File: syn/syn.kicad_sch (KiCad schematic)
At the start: 47 parts, among them J1 AudioJack2, Q1 BC546, SW1 Range, SW3 Wave, SW4 Wave, SW5 Mod, SW6 SW_Push_SPDT, U1 TL074, U2 LM741

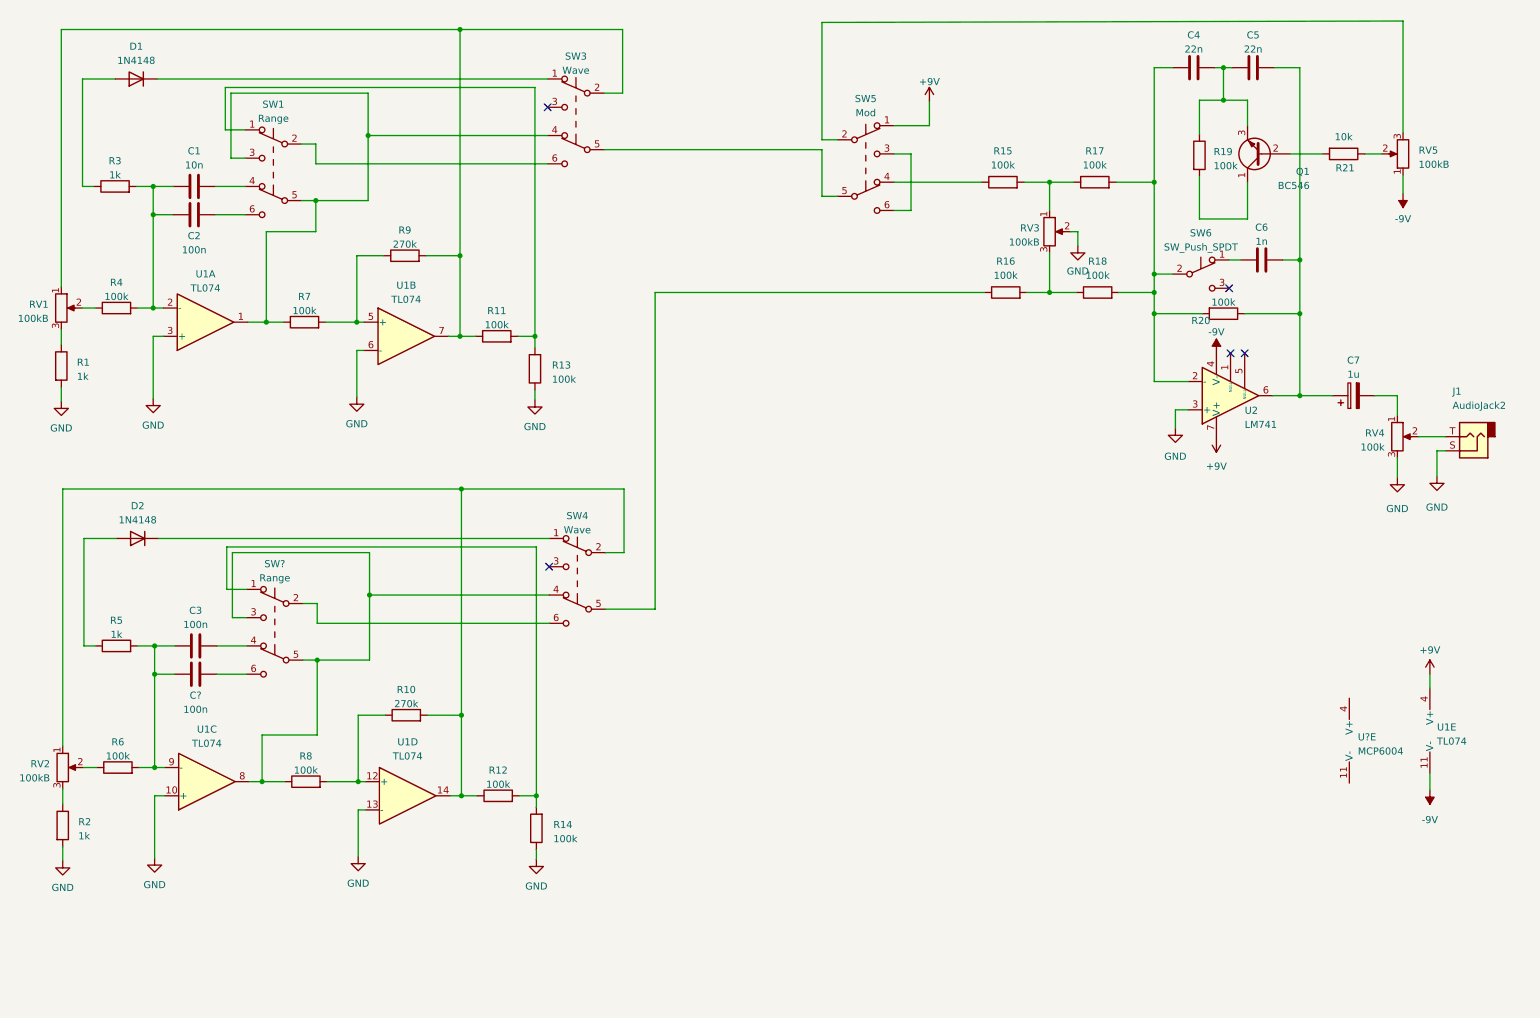
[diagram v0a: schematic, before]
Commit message: structure
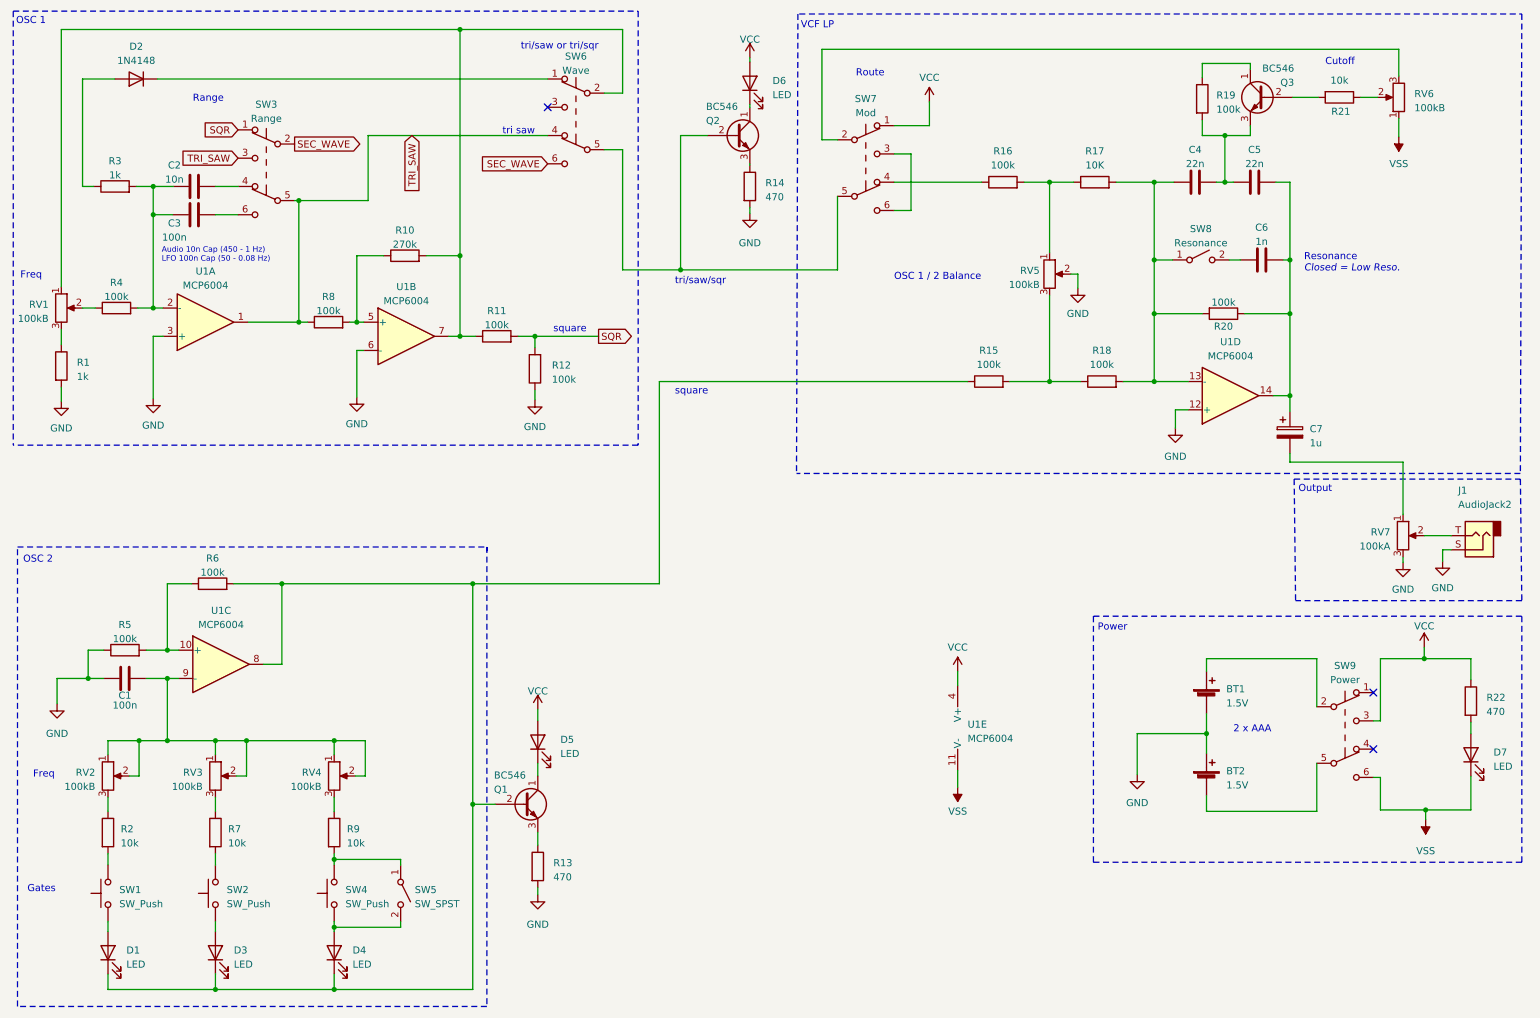
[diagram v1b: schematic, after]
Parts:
- removed C3, C?: 100n, symbol Device:C
- removed D2: 1N4148, Diode_THT:D_DO-35_SOD27_P7.62mm_Horizontal, symbol Diode:1N4148
- removed R10: 270k, symbol Device:R
- removed R12, R8: 100k, symbol Device:R
- removed SW4: Wave, symbol Switch:SW_Push_DPDT
- removed SW6: SW_Push_SPDT, symbol Switch:SW_Push_SPDT
- removed SW?: Range, symbol Switch:SW_Push_DPDT
- removed U1: TL074, symbol Amplifier_Operational:TL074
- removed U2: LM741, symbol Amplifier_Operational:LM741
- removed U?: MCP6004, symbol Amplifier_Operational:MCP6004
- added BT1, BT2: 1.5V, Battery:BatteryHolder_Keystone_2466_1xAAA, symbol Device:Battery_Cell
- added C1: 100n, symbol Device:C
- added D1, D3, D4, D5, D6, D7: LED, symbol Device:LED
- added Q1, Q2: BC546, Package_TO_SOT_THT:TO-92_Inline, symbol Transistor_BJT:BC546
- added R13, R22: 470, symbol Device:R
- added R7, R9: 10k, symbol Device:R
- added RV3, RV4: 100kB, symbol Device:R_Potentiometer
- added SW1, SW2, SW4: SW_Push, symbol Switch:SW_Push
- added SW5: SW_SPST, symbol Switch:SW_SPST
- added SW8: Resonance, symbol Switch:SW_SPST
- added SW9: Power, symbol Switch:SW_Push_DPDT
- added U1: MCP6004, symbol Amplifier_Operational:MCP6004
- R14: value 100k -> 470
- R17: value 100k -> 10K
- R2: value 1k -> 10k
- R5: value 1k -> 100k
- RV7: renamed from RV4; value 100k -> 100kA
- renumbered C1 to C2, C2 to C3, D1 to D2, Q1 to Q3, R9 to R10, R13 to R12, R16 to R15, R15 to R16, R7 to R8, RV3 to RV5, RV5 to RV6, SW1 to SW3, SW3 to SW6, SW5 to SW7
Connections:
- net GND: now also R14.2, R5.1, BT1.2 (-), BT2.1 (+), C1.1, R13.2, U1.12 (+), U1.3 (+), U1.6 (-); no longer R14.1, R2.2
- net at C2.1, C3.1, R3.2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: now also U1.2 (-)
- net TRI_SAW: now reaches R8.1, SW3.3 (C), SW3.5 (B), SW6.4 (A)
- net TRI_SAW: now also U1.1
- net at R5.2: now also R6.1, U1.10 (+); no longer R6.2
- net at C6.1: now also SW8.2 (B)
- net at C5.2, C6.2, C7.1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: now also U1.14
- net at RV2.1: now also RV2.2, C1.2, RV3.1, RV3.2, RV4.1, RV4.2, U1.9 (-)
- net at C4.1, R17.2, R18.2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: now also SW8.1 (A), U1.13 (-)
- net at R10.1, R8.2: now also U1.5 (+)
- net at R10.2, R11.1, RV1.1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: now also U1.7
- net at R15.1: now also R6.2, D1.1 (K), D3.1 (K), D4.1 (K), Q1.2 (B), U1.8
- net at SW6.5 (B), SW7.5 (B): now also Q2.2 (B)
- net SEC_WAVE: now reaches SW3.2 (B), SW6.6 (C)
- net SQR: now reaches R11.2, R12.2, SW3.1 (A)
- net at C4.2, C5.1, Q3.3 (E): now also R19.2; no longer R19.1
- net at Q3.1 (C): now also R19.1; no longer R19.2
- net +9V renamed VCC
- net VCC: now also D5.2 (A), D6.2 (A), R22.1, SW9.3 (C), U1.4 (V+)
- net -9V renamed VSS
- net VSS: now also D7.1 (K), SW9.6 (C), U1.11 (V-)
- new net: D5.1 (K), Q1.1 (C)
- new net: Q1.3 (E), R13.1
- new net: D4.2 (A), SW4.1, SW5.2 (B)
- new net: R9.2, SW4.2, SW5.1 (A)
- new net: D7.2 (A), R22.2
- new net: D1.2 (A), SW1.1
- new net: R2.2, SW1.2
- new net: D6.1 (K), Q2.1 (C)
- new net: BT1.1 (+), SW9.2 (B)
- new net: BT2.2 (-), SW9.5 (B)
- new net: R9.1, RV4.3
- new net: D3.2 (A), SW2.1
- new net: R7.1, RV3.3
- new net: R7.2, SW2.2
- new net: Q2.3 (E), R14.1
- no-connect marks 5 -> 3
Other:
- note added: "2 x AAA"
- note added: "Audio 10n Cap (450 - 1 Hz) LFO 100n Cap (50 - 0.08 Hz)"
- note added: "Closed = Low Reso."
- note added: "Cutoff"
- note added: "Freq"
- note added: "Gates"
- note added: "OSC 1"
- note added: "OSC 1 / 2 Balance"
- note added: "OSC 2"
- note added: "Output"
- note added: "Power"
- note added: "Range"
- note added: "Resonance"
- note added: "Route"
- note added: "VCF LP"
- note added: "square"
- note added: "tri saw"
- note added: "tri/saw or tri/sqr"
- note added: "tri/saw/sqr"
- moved on the sheet: C4, C5, C7, J1, Q3, R15, R18, R19, R21, R8, RV5, RV6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
